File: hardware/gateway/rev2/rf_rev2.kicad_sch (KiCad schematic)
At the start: 26 parts, among them IC2 CC1101RGPR, Y1 NX3225GA-26.000M-STD-CRG-2

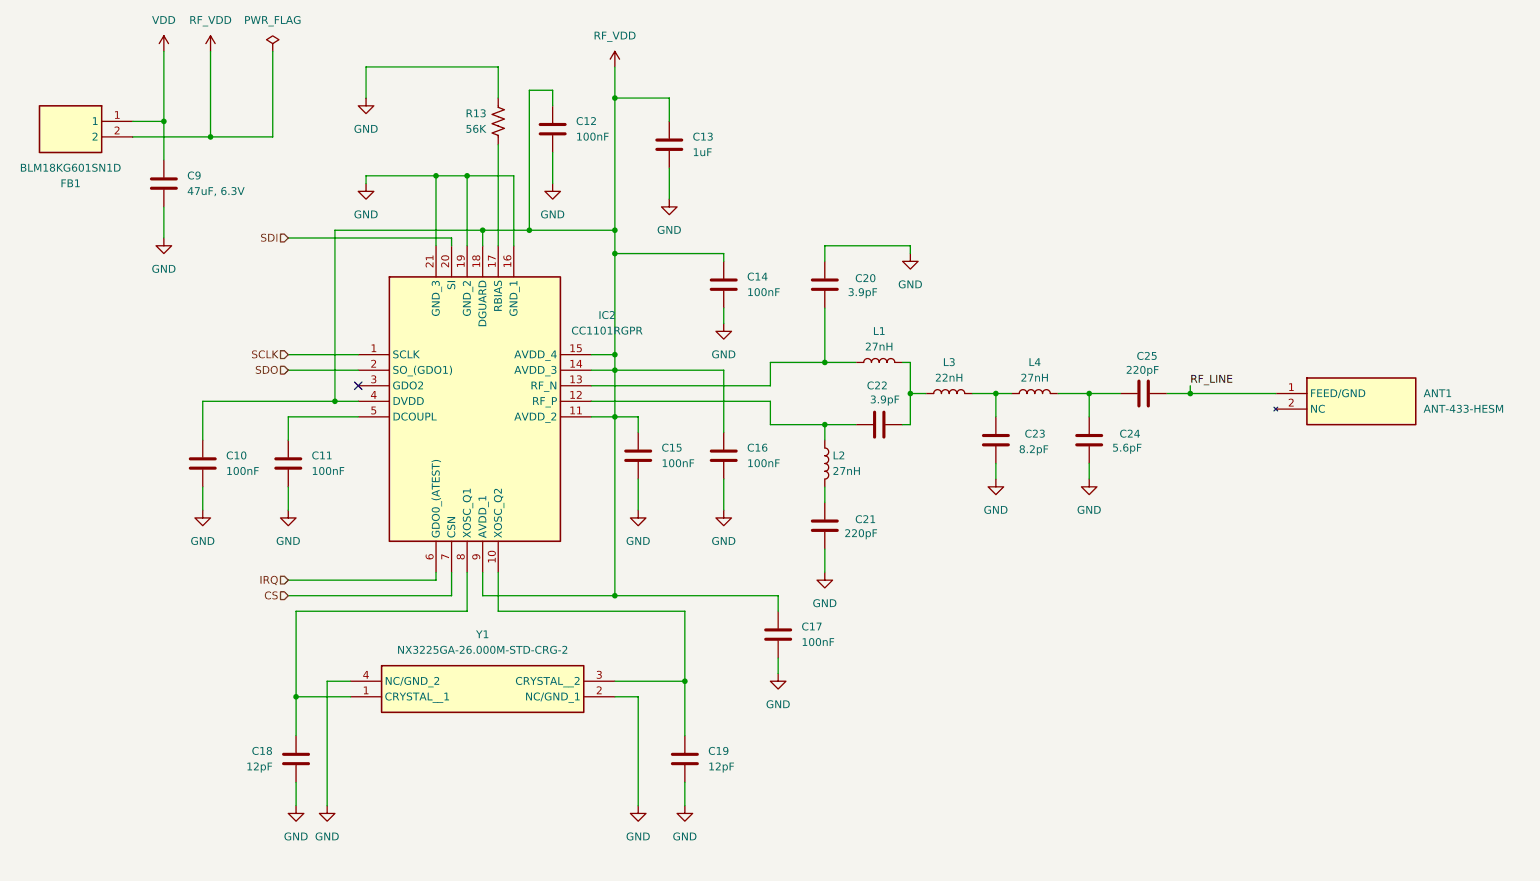
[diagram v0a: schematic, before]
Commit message: EG-59 Schematic with the needed components, plus PCB.
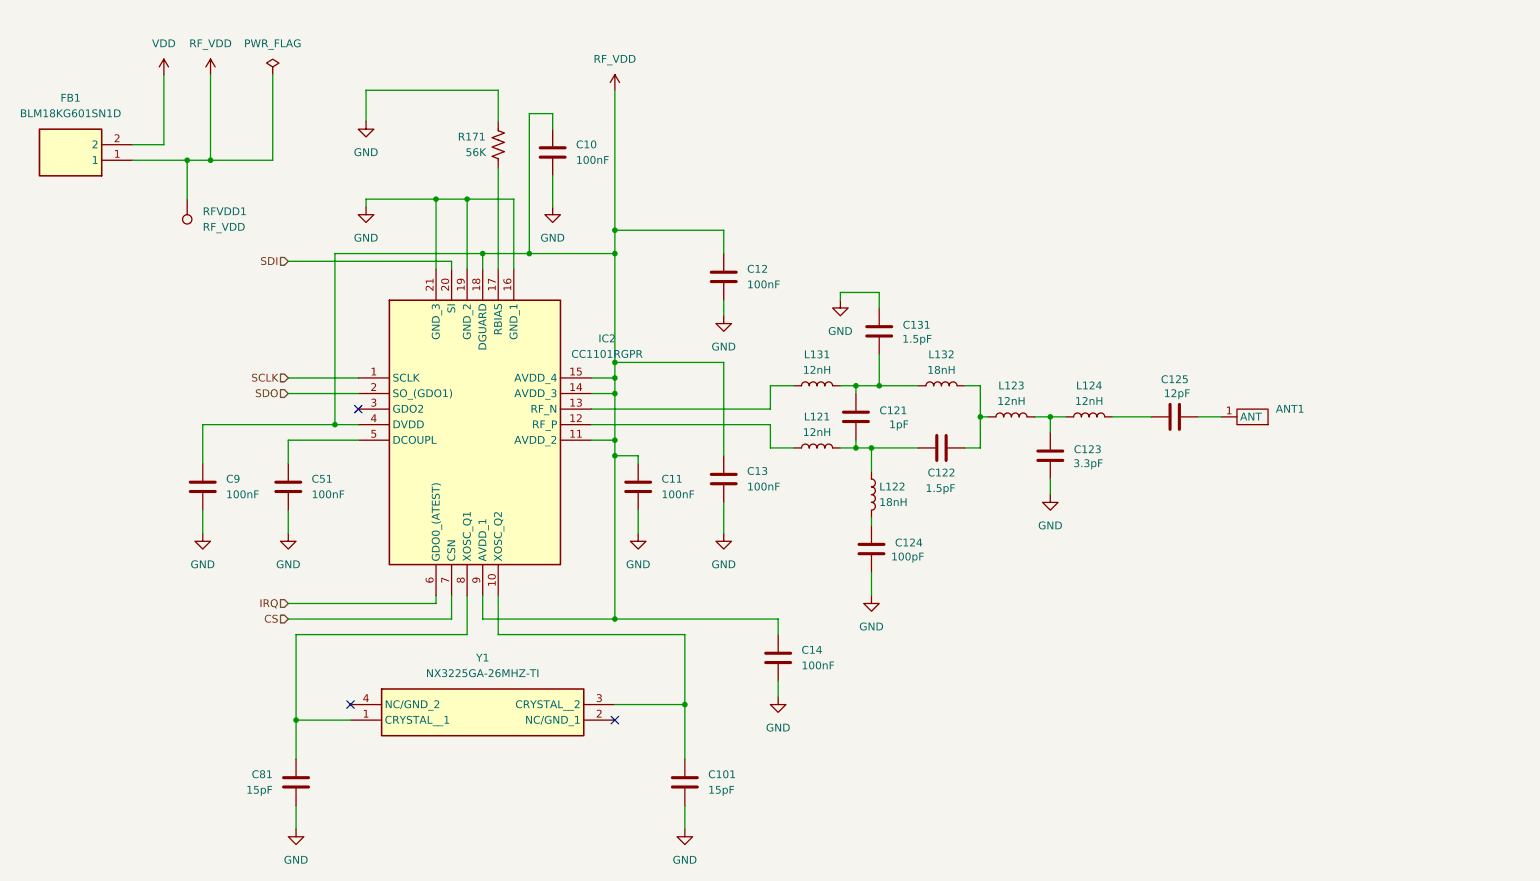
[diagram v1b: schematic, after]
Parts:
- removed ANT1: ANT-433-HESM, MyParts:ANT433HESM, symbol ANT-433-HESM:ANT-433-HESM
- removed C15, C16, C17: 100nF, Capacitor_SMD:C_0402_1005Metric, symbol Device:C
- removed C18, C19: 12pF, Capacitor_SMD:C_0402_1005Metric, symbol Device:C
- removed C20, C22: 3.9pF, Capacitor_SMD:C_0402_1005Metric, symbol Device:C
- removed C21, C25: 220pF, Capacitor_SMD:C_0402_1005Metric, symbol Device:C
- removed C23: 8.2pF, Capacitor_SMD:C_0402_1005Metric, symbol Device:C
- removed C24: 5.6pF, Capacitor_SMD:C_0402_1005Metric, symbol Device:C
- removed L1, L2, L4: 27nH, Inductor_SMD:L_0402_1005Metric, symbol Device:L
- removed L3: 22nH, Inductor_SMD:L_0402_1005Metric, symbol Device:L
- removed R13: 56K, Resistor_SMD:R_0402_1005Metric, symbol Device:R_US
- added ANT1: (no value), MyParts:Antenna_hole, symbol antenna_hole:Antenna_Hole
- added C101, C81: 15pF, Capacitor_SMD:C_0402_1005Metric, symbol Device:C
- added C121: 1pF, Capacitor_SMD:C_0402_1005Metric, symbol Device:C
- added C122, C131: 1.5pF, Capacitor_SMD:C_0402_1005Metric, symbol Device:C
- added C123: 3.3pF, Capacitor_SMD:C_0402_1005Metric, symbol Device:C
- added C124: 100pF, Capacitor_SMD:C_0402_1005Metric, symbol Device:C
- added C125: 12pF, Capacitor_SMD:C_0402_1005Metric, symbol Device:C
- added C51: 100nF, Capacitor_SMD:C_0402_1005Metric, symbol Device:C
- added L121, L123, L124, L131: 12nH, Inductor_SMD:L_0402_1005Metric, symbol Device:L
- added L122, L132: 18nH, Inductor_SMD:L_0402_1005Metric, symbol Device:L
- added R171: 56K, Resistor_SMD:R_0402_1005Metric, symbol Device:R_US
- added RFVDD1: RF_VDD, TestPoint:TestPoint_Pad_D1.0mm, symbol Connector:TestPoint
- C10, C11, C12, C14: Manufacturer Yageo -> (none); Manufacturer Part Number CC0402KRX7R7BB104 -> (none); Manufacturer_Name (none) -> Yageo; Manufacturer_Part_Number (none) -> CC0402KRX7R7BB104; Mouser Price/Stock (none) -> https://pt.mouser.com/ProductDetail/YAGEO/CC0402KRX7R7BB104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; Supplier Link https://pt.mouser.com/ProductDetail/YAGEO/CC0402KRX7R7BB104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 -> (none)
- C13: value 1uF -> 100nF; Manufacturer Murata -> (none); Manufacturer Part Number GXT155R60J105KE01D -> (none); Manufacturer_Name (none) -> Yageo; Manufacturer_Part_Number (none) -> CC0402KRX7R7BB104; Mouser Part Number 81-GXT155R60J105KE1D -> 603-CC402KRX7R7BB104; Mouser Price/Stock (none) -> https://pt.mouser.com/ProductDetail/YAGEO/CC0402KRX7R7BB104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; Supplier Link https://pt.mouser.com/ProductDetail/Murata-Electronics/GXT1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 -> (none)
- C9: value 47uF, 6.3V -> 100nF; footprint Capacitor_SMD:C_1206_3216Metric -> Capacitor_SMD:C_0402_1005Metric; Manufacturer TAYO YUDEN -> (none); Manufacturer Part Number JMK316BJ476MD-T -> (none); Manufacturer_Name (none) -> Yageo; Manufacturer_Part_Number (none) -> CC0402KRX7R7BB104; Mouser Part Number 963-JMK316BJ476MD-T -> 603-CC402KRX7R7BB104; Mouser Price/Stock (none) -> https://pt.mouser.com/ProductDetail/YAGEO/CC0402KRX7R7BB104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; Supplier Link https://pt.mouser.com/ProductDetail/TAIYO-YUDEN/JMK316BJ476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 -> (none)
- FB1: Manufacturer Murata Electronics -> (none); Manufacturer_Name (none) -> Murata Electronics; Mouser Price/Stock (none) -> https://www.mouser.co.uk/ProductDetail/Murata-Electronics/B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; Supplier Link https://www.mouser.co.uk/ProductDetail/Murata-Electronics/B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 -> (none)
- IC2: Manufacturer Texas Instruments -> (none); Manufacturer_Name (none) -> Texas Instruments; Mouser Price/Stock (none) -> https://www.mouser.co.uk/ProductDetail/Texas-Instruments/CC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; Supplier Link https://www.mouser.co.uk/ProductDetail/Texas-Instruments/CC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 -> (none)
- Y1: value NX3225GA-26.000M-STD-CRG-2 -> NX3225GA-26MHZ-TI; Manufacturer NDK -> (none); Manufacturer Part Number NX3225GA-26.000M-STD-CRG-2 -> NX3225GA-26MHZ-TI; Manufacturer_Name (none) -> NDK; Mouser Part Number 344-NX3225GA26MSTRG2 -> 344-NX3225GA26MHZTI; Mouser Price/Stock (none) -> https://pt.mouser.com/en/ProductDetail/NDK/CG01972-26M?qs=T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; Supplier Link https://www.mouser.co.uk/ProductDetail/NDK/NX3225GA-26.000M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 -> (none)
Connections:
- net GND: now also C101.2, C123.1, C124.1, C131.2, C51.2, C81.2, R171.2; no longer Y1.2 (NC/GND_1), Y1.4 (NC/GND_2)
- net RF_VDD: now also C11.1, C9.1, FB1.1, RFVDD1.1; no longer FB1.2
- net VDD: now also FB1.2; no longer C9.1, FB1.1
- net at IC2.13 (RF_N): now also L131.1
- net at IC2.12 (RF_P): now also L121.1
- net at IC2.17 (RBIAS): now also R171.1
- net at IC2.10 (XOSC_Q2), Y1.3 (CRYSTAL__2): now also C101.1
- net at IC2.5 (DCOUPL): now also C51.1; no longer C11.1
- net at IC2.8 (XOSC_Q1), Y1.1 (CRYSTAL__1): now also C81.1
- new net: C121.2, C131.1, L131.2, L132.1
- new net: C123.2, L123.2, L124.1
- new net: C125.1, L124.2
- new net: C124.2, L122.2
- new net: C122.2, L123.1, L132.2
- new net: C121.1, C122.1, L121.2, L122.1
- new net: ANT1.1 (ANT), C125.2
- no-connect marks 1 -> 3
